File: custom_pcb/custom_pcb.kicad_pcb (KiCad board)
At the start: 2 copper layers, 285 x 152 mm, 316 parts, among them J1 USB_mini_micro_B, K0 KEYSW, K1 KEYSW, K10 KEYSW, K11 KEYSW, K12 KEYSW, K13 KEYSW, K14 KEYSW, K15 KEYSW, K16 KEYSW, K17 KEYSW, K18 KEYSW, K19 KEYSW, K2 KEYSW, K20 KEYSW, K21 KEYSW, K22 KEYSW, K23 KEYSW, K24 KEYSW, K25 KEYSW, K26 KEYSW, K27 KEYSW, K28 KEYSW, K29 KEYSW, K3 KEYSW, K30 KEYSW, K31 KEYSW, K32 KEYSW, K33 KEYSW, K34 KEYSW, K35 KEYSW, K36 KEYSW, K37 KEYSW, K38 KEYSW, K39 KEYSW, K4 KEYSW, K40 KEYSW, K41 KEYSW, K42 KEYSW, K43 KEYSW, K44 KEYSW, K45 KEYSW, K46 KEYSW, K47 KEYSW, K48 KEYSW, K49 KEYSW, K5 KEYSW, K50 KEYSW, K51 KEYSW, K52 KEYSW, K53 KEYSW, K54 KEYSW, K55 KEYSW, K56 KEYSW, K57 KEYSW, K58 KEYSW, K59 KEYSW, K6 KEYSW, K60 KEYSW, K63 KEYSW, K64 KEYSW, K65 KEYSW, K66 KEYSW, K67 KEYSW, K68 KEYSW, K69 KEYSW, K7 KEYSW, K70 KEYSW, K71 KEYSW, K72 KEYSW, K73 KEYSW, K74 KEYSW, K75 KEYSW, K76 KEYSW, K77 KEYSW, K78 KEYSW, K79 KEYSW, K8 KEYSW, K80 KEYSW, K81 KEYSW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

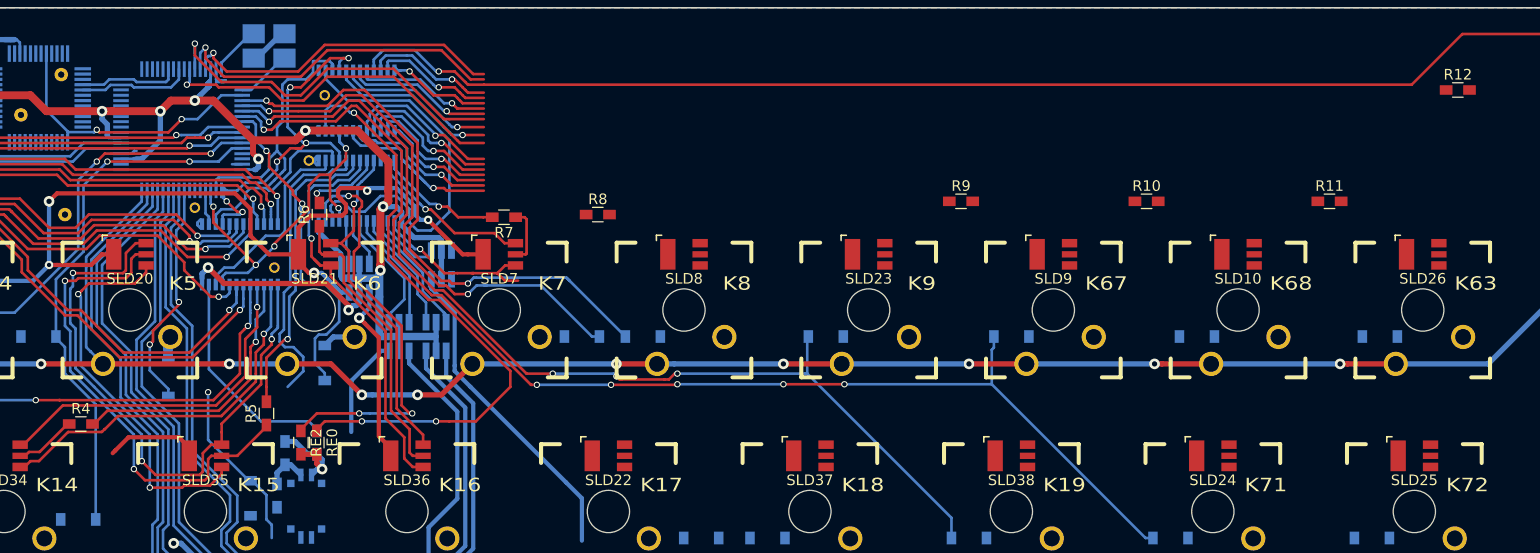
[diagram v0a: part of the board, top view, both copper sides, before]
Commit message: more tweaks
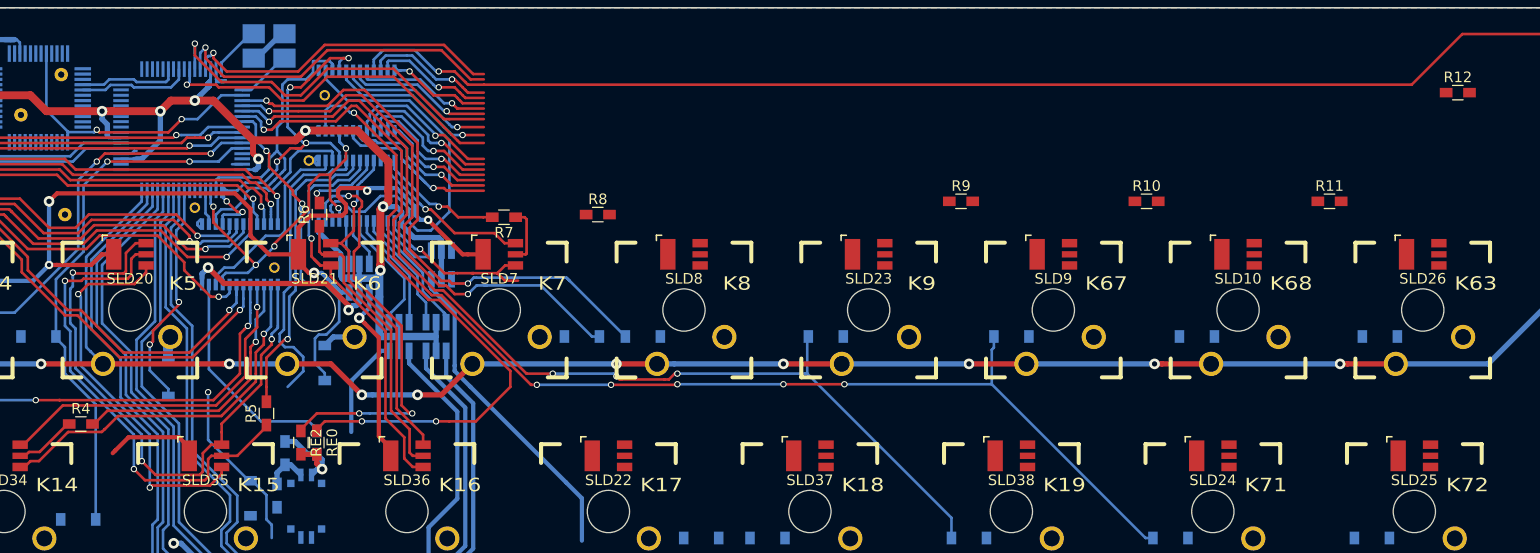
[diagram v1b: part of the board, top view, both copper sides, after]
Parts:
- moved R12 0.25 mm to (256.1, 33.5)
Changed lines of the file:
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@@
     (thickness 1.6)
     (drawings 6)
-    (tracks 1961)
+    (tracks 1958)
     (zones 0)
     (modules 316)
@@
   )
   (module Resistors_SMD:R_0603_HandSoldering (layer F.Cu)
-    (at 256.1 33.25)
+    (at 256.1 33.5)
     (descr "Resistor SMD 0603, hand soldering")
     (tags "resistor 0603")
@@
   (segment (start 122.364999 67.385001) (end 125 64.75) (width 0.25) (layer F.Cu) (net 122))
   (segment (start 125 64.75) (end 125.15 64.75) (width 0.25) (layer F.Cu) (net 122))
+  (segment (start 124.75 51.25) (end 126.3 51.25) (width 0.25) (layer F.Cu) (net 123))
+  (segment (start 126.5 51.05) (end 130.65 51.05) (width 0.25) (layer F.Cu) (net 123))
+  (segment (start 130.65 51.05) (end 131 50.7) (width 0.25) (layer F.Cu) (net 123))
+  (segment (start 131 50.7) (end 131 49.175) (width 0.25) (layer F.Cu) (net 123))
+  (segment (start 131 49.175) (end 131.425 48.75) (width 0.25) (layer F.Cu) (net 123))
+  (segment (start 126.3 51.25) (end 126.5 51.05) (width 0.25) (layer F.Cu) (net 123))
+  (segment (start 131.425 48.75) (end 132.4 48.75) (width 0.25) (layer F.Cu) (net 123))
   (via (at 131.25 69) (size 0.6) (drill 0.4) (layers F.Cu B.Cu) (net 123))
   (segment (start 132.3 70.05) (end 131.25 69) (width 0.25) (layer F.Cu) (net 123))
@@
   (segment (start 124.75 51.25) (end 124.75 55.5) (width 0.25) (layer B.Cu) (net 123))
   (segment (start 124.75 55.5) (end 125.25 56) (width 0.25) (layer B.Cu) (net 123))
-  (segment (start 130.5 51) (end 126 51) (width 0.25) (layer F.Cu) (net 123))
-  (segment (start 131 49.175) (end 131 50.5) (width 0.25) (layer F.Cu) (net 123))
-  (segment (start 130.5 51) (end 131 50.5) (width 0.25) (layer F.Cu) (net 123))
   (segment (start 139.525 67.75) (end 138.55 67.75) (width 0.25) (layer F.Cu) (net 123))
   (segment (start 138.55 67.75) (end 138.25 68.05) (width 0.25) (layer F.Cu) (net 123))
-  (segment (start 125.75 51.25) (end 124.75 51.25) (width 0.25) (layer F.Cu) (net 123))
-  (segment (start 126 51) (end 125.75 51.25) (width 0.25) (layer F.Cu) (net 123))
   (via (at 124.75 51.25) (size 0.6) (drill 0.4) (layers F.Cu B.Cu) (net 123))
-  (segment (start 132.4 48.75) (end 131.425 48.75) (width 0.25) (layer F.Cu) (net 123))
-  (segment (start 131.425 48.75) (end 131 49.175) (width 0.25) (layer F.Cu) (net 123))
   (segment (start 148.75 48.5) (end 148.75 46.1) (width 0.25) (layer F.Cu) (net 124))
   (segment (start 149.81667 48.75) (end 150.79167 48.75) (width 0.25) (layer F.Cu) (net 124))
@@
   (via (at 142.875 53.728357) (size 0.6) (drill 0.4) (layers F.Cu B.Cu) (net 141))
   (segment (start 142.875 51.6) (end 142.875 53.728357) (width 0.25) (layer B.Cu) (net 141))
-  (segment (start 138.425 70.55) (end 136 70.55) (width 0.25) (layer F.Cu) (net 142))
-  (segment (start 132.75 70.75) (end 135.8 70.75) (width 0.25) (layer F.Cu) (net 142))
-  (segment (start 135.8 70.75) (end 136 70.55) (width 0.25) (layer F.Cu) (net 142))
-  (via (at 132.75 70.75) (size 0.6) (drill 0.4) (layers F.Cu B.Cu) (net 142))
+  (segment (start 132.4 49.8) (end 132.4 50.45) (width 0.25) (layer F.Cu) (net 142))
+  (segment (start 132.4 50.45) (end 131.3 51.55) (width 0.25) (layer F.Cu) (net 142))
+  (segment (start 131.3 51.55) (end 126.95 51.55) (width 0.25) (layer F.Cu) (net 142))
+  (segment (start 126.95 51.55) (end 126 52.5) (width 0.25) (layer F.Cu) (net 142))
   (segment (start 139.525 68.8) (end 139.525 69.45) (width 0.25) (layer F.Cu) (net 142))
   (segment (start 139.525 69.45) (end 138.425 70.55) (width 0.25) (layer F.Cu) (net 142))
+  (segment (start 138.425 70.55) (end 132.95 70.55) (width 0.25) (layer F.Cu) (net 142))
+  (segment (start 132.95 70.55) (end 132.75 70.75) (width 0.25) (layer F.Cu) (net 142))
+  (via (at 132.75 70.75) (size 0.6) (drill 0.4) (layers F.Cu B.Cu) (net 142))
   (segment (start 132.75 65.75) (end 132.75 70.75) (width 0.25) (layer B.Cu) (net 142))
   (segment (start 129.5 62.5) (end 132.75 65.75) (width 0.25) (layer B.Cu) (net 142))
@@
   (segment (start 147.215359 59.784641) (end 145.75 61.25) (width 0.25) (layer B.Cu) (net 142))
   (segment (start 126 52.5) (end 126.25 52.75) (width 0.25) (layer B.Cu) (net 142))
-  (segment (start 131.35 51.5) (end 127 51.5) (width 0.25) (layer F.Cu) (net 142))
-  (segment (start 126 52.5) (end 126.299999 52.200001) (width 0.25) (layer F.Cu) (net 142))
-  (segment (start 126.299999 52.200001) (end 127 51.5) (width 0.25) (layer F.Cu) (net 142))
   (via (at 126 52.5) (size 0.6) (drill 0.4) (layers F.Cu B.Cu) (net 142))
-  (segment (start 132.4 50.45) (end 131.35 51.5) (width 0.25) (layer F.Cu) (net 142))
-  (segment (start 132.4 49.8) (end 132.4 50.45) (width 0.25) (layer F.Cu) (net 142))
+  (segment (start 132.4 47.7) (end 131.425 47.7) (width 0.25) (layer F.Cu) (net 143))
+  (segment (start 131.425 47.7) (end 130.5 48.625) (width 0.25) (layer F.Cu) (net 143))
+  (segment (start 130.5 48.625) (end 130.5 50.35) (width 0.25) (layer F.Cu) (net 143))
+  (segment (start 130.5 50.35) (end 130.3 50.55) (width 0.25) (layer F.Cu) (net 143))
+  (segment (start 130.3 50.55) (end 125.578367 50.55) (width 0.25) (layer F.Cu) (net 143))
+  (segment (start 125.578367 50.55) (end 125.493357 50.46499) (width 0.25) (layer F.Cu) (net 143))
+  (segment (start 125.25 55.25) (end 125.25 52) (width 0.25) (layer B.Cu) (net 143))
+  (segment (start 125.493357 50.889254) (end 125.493357 50.46499) (width 0.25) (layer B.Cu) (net 143))
+  (segment (start 125.493357 51.756643) (end 125.493357 50.889254) (width 0.25) (layer B.Cu) (net 143))
+  (segment (start 125.25 52) (end 125.493357 51.756643) (width 0.25) (layer B.Cu) (net 143))
+  (segment (start 125.75 55.75) (end 125.25 55.25) (width 0.25) (layer B.Cu) (net 143))
+  (segment (start 132 68.25) (end 132 65.75) (width 0.25) (layer B.Cu) (net 143))
+  (segment (start 132 65.75) (end 125.75 59.5) (width 0.25) (layer B.Cu) (net 143))
+  (via (at 125.493357 50.46499) (size 0.6) (drill 0.4) (layers F.Cu B.Cu) (net 143))
+  (segment (start 125.75 59.5) (end 125.75 55.75) (width 0.25) (layer B.Cu) (net 143))
   (segment (start 137.75 69.25) (end 137.75 67.5) (width 0.25) (layer F.Cu) (net 143))
   (segment (start 137.45 69.55) (end 137.75 69.25) (width 0.25) (layer F.Cu) (net 143))
@@
   (segment (start 132 68.25) (end 133.3 69.55) (width 0.25) (layer F.Cu) (net 143))
   (via (at 132 68.25) (size 0.6) (drill 0.4) (layers F.Cu B.Cu) (net 143))
-  (segment (start 132 65.75) (end 132 68.25) (width 0.25) (layer B.Cu) (net 143))
-  (segment (start 127.5 61.25) (end 132 65.75) (width 0.25) (layer B.Cu) (net 143))
-  (segment (start 125.75 55.75) (end 125.75 59.5) (width 0.25) (layer B.Cu) (net 143))
-  (segment (start 125.75 59.5) (end 127.5 61.25) (width 0.25) (layer B.Cu) (net 143))
   (segment (start 144.825 51.6) (end 144.825 55.5) (width 0.25) (layer B.Cu) (net 143))
   (segment (start 144.825 55.5) (end 144.825 55.675) (width 0.25) (layer B.Cu) (net 143))
@@
   (segment (start 139.525 64.725) (end 143.25 61) (width 0.25) (layer F.Cu) (net 143))
   (segment (start 143.25 61) (end 143.25 58.25) (width 0.25) (layer F.Cu) (net 143))
-  (segment (start 125.5 50.5) (end 125.5 51.75) (width 0.25) (layer B.Cu) (net 143))
-  (segment (start 125.5 51.75) (end 125.25 52) (width 0.25) (layer B.Cu) (net 143))
-  (segment (start 125.25 52) (end 125.25 55.25) (width 0.25) (layer B.Cu) (net 143))
-  (segment (start 125.25 55.25) (end 125.75 55.75) (width 0.25) (layer B.Cu) (net 143))
   (segment (start 139.525 65.525) (end 139.525 64.725) (width 0.25) (layer F.Cu) (net 143))
   (segment (start 138.55 66.7) (end 137.75 67.5) (width 0.25) (layer F.Cu) (net 143))
-  (segment (start 132.4 47.7) (end 131.425 47.7) (width 0.25) (layer F.Cu) (net 143))
-  (segment (start 130.224999 50.525001) (end 125.775001 50.525001) (width 0.25) (layer F.Cu) (net 143))
-  (segment (start 131.425 47.7) (end 130.5 48.625) (width 0.25) (layer F.Cu) (net 143))
-  (segment (start 125.775001 50.525001) (end 125.75 50.5) (width 0.25) (layer F.Cu) (net 143))
-  (segment (start 130.5 48.625) (end 130.5 50.25) (width 0.25) (layer F.Cu) (net 143))
-  (segment (start 130.5 50.25) (end 130.224999 50.525001) (width 0.25) (layer F.Cu) (net 143))
-  (segment (start 125.75 50.5) (end 125.5 50.5) (width 0.25) (layer F.Cu) (net 143))
-  (via (at 125.5 50.5) (size 0.6) (drill 0.4) (layers F.Cu B.Cu) (net 143))
   (segment (start 139.525 65.525) (end 139.525 66.7) (width 0.25) (layer F.Cu) (net 143))
   (segment (start 139.525 66.7) (end 138.55 66.7) (width 0.25) (layer F.Cu) (net 143))
